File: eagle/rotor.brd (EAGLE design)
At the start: 72.1 x 80 mm, 53 parts, among them IC1 TXS0108, IC2 7815TV, J1 PL9823, J2 pwr2, J3 Power, J4 Antenna, J5 Power, J6 CCW, J7 Brake, J8 CW, J9 Rotor-Pwr-LED, Q1 2N2907, T1 2N2222, U1 RPi Header, U2 ADS1115, U3 LMV358

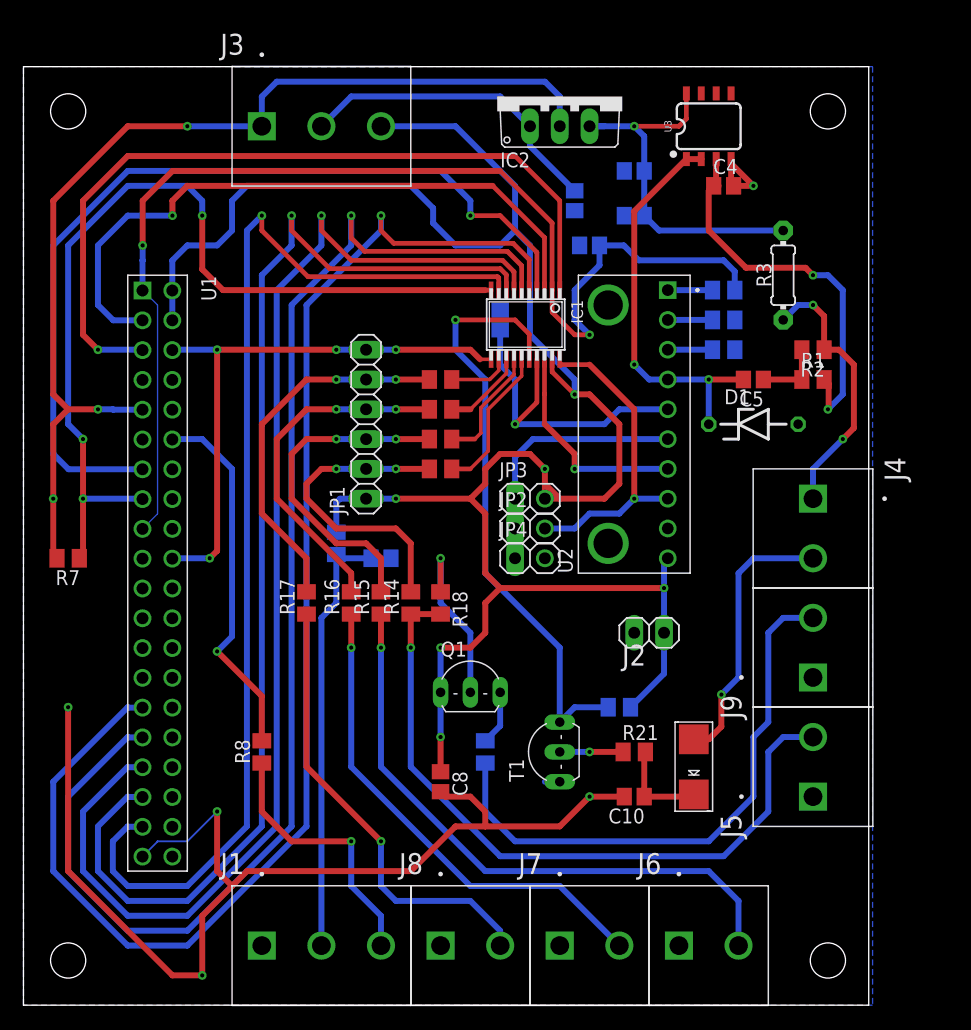
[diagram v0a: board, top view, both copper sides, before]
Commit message: eagle
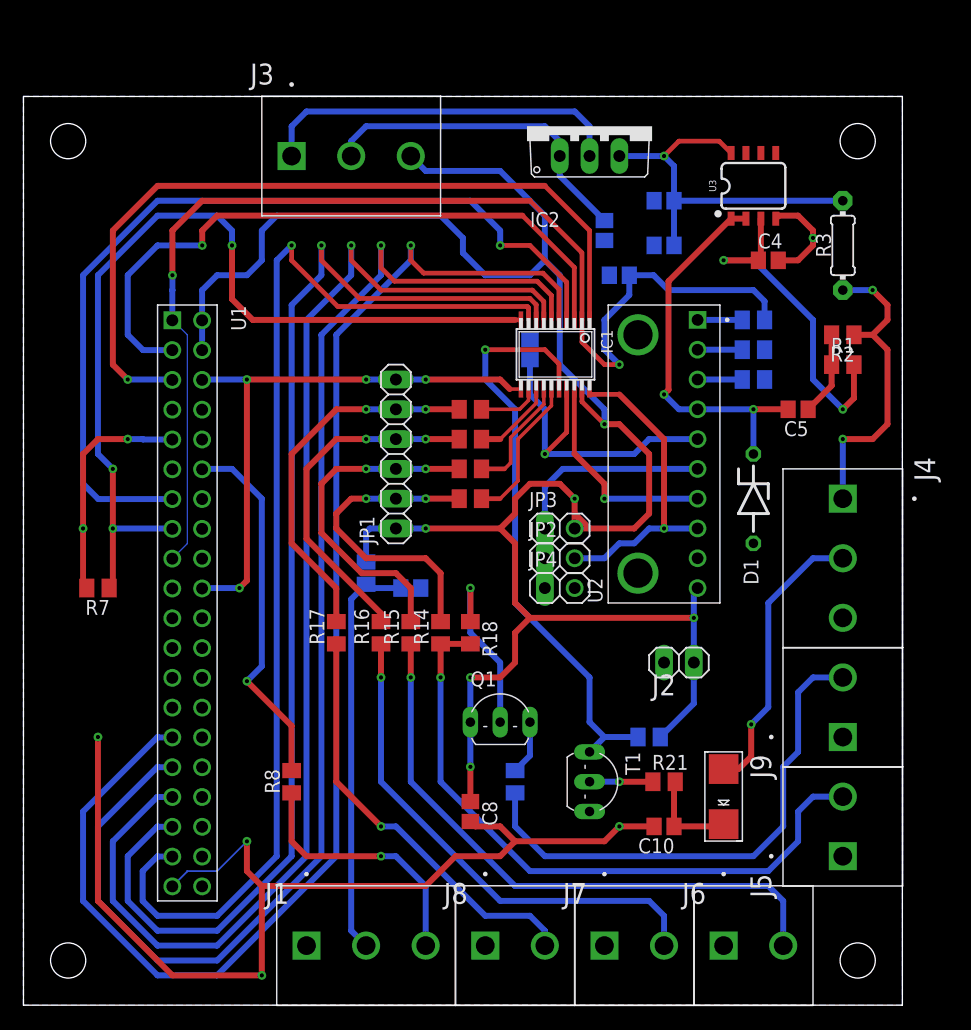
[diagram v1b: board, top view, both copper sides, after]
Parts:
- J4: device TB004-508-02BE:CUI_TB004-508-02BE -> TB004-508-03BE:CUI_TB004-508-03BE
- Q1, T1: device test:TO92-EBC-OVAL -> test:TO92-CBE-OVAL
- R3: value 1100 -> 1100 Ω
- moved C4 7.41 mm to (63.5, 63.5)
- moved U3 6.35 mm to (62.2, 69.8)
- moved D1 6.35 mm to (62.2, 43.2), turned to 270 degrees
- moved J5 5.68 mm to (69.8, 12.7)
- moved J9 5.68 mm to (69.8, 22.9)
- moved R3 5.68 mm to (69.8, 64.8)
- moved T1 5.68 mm to (49.5, 19.1), turned to 270 degrees
- moved C5 4.58 mm to (66.0, 50.8)
- moved J7 3.81 mm to (49.5, 5.08)
- moved J1 3.81 mm to (24.1, 5.08)
- moved J6 3.81 mm to (59.7, 5.08)
- moved J8 3.81 mm to (39.4, 5.08)
- moved C1 3.59 mm to (54.6, 68.6)
- moved C3 3.59 mm to (54.6, 64.8)
- moved J3 3.59 mm to (22.9, 72.4)
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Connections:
- net +5V: now also Q1.C; no longer Q1.E
- net GND: now also J4.3
- net N$8: now also Q1.E; no longer Q1.C
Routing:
- net GND: track 241.7 -> 199.1 mm, vias 12 -> 11
- net N$1: track 33.7 -> 29.2 mm
- net SW1-POWER: track 60.2 -> 55.9 mm
- net ROTOR-PWR-LED-SOURCE: track 48.5 -> 44.1 mm
- net ROOF-3: track 23.2 -> 26.6 mm
- net SW4-CW: track 38.8 -> 36.1 mm
- net PL9823-SOURCE: track 37.0 -> 35.3 mm
- net +24: track 27.0 -> 28.5 mm
- net N$3: track 5.82 -> 7.18 mm
- net ROOF-4: track 23.4 -> 24.4 mm
- net SW3-BRAKE: track 42.2 -> 43.2 mm
- net CH0: track 34.3 -> 33.5 mm
- net POWER-OUT: track 51.6 -> 50.8 mm
- net +15V: track 32.3 -> 32.8 mm
- net SW2-CCW: track 52.0 -> 51.5 mm
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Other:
- board size 72.1 x 80 mm -> 74.9 x 77.5 mm
